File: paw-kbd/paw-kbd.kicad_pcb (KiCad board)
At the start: 2 copper layers, 30 parts, among them J1 OLED, J2 MJ-4PP-9, SW10 SW_PUSH, SW11 SW_PUSH, SW12 SW_PUSH, SW13 SW_PUSH, SW14 SW_PUSH, SW15 SW_PUSH, SW16 SW_PUSH, SW17 SW_PUSH, SW18 SW_PUSH, SW22 SW_PUSH, SW4 SW_PUSH, SW5 SW_PUSH, SW6 SW_PUSH, SW7 SW_PUSH, SW8 SW_PUSH, SW9 SW_PUSH, U1 ProMicro

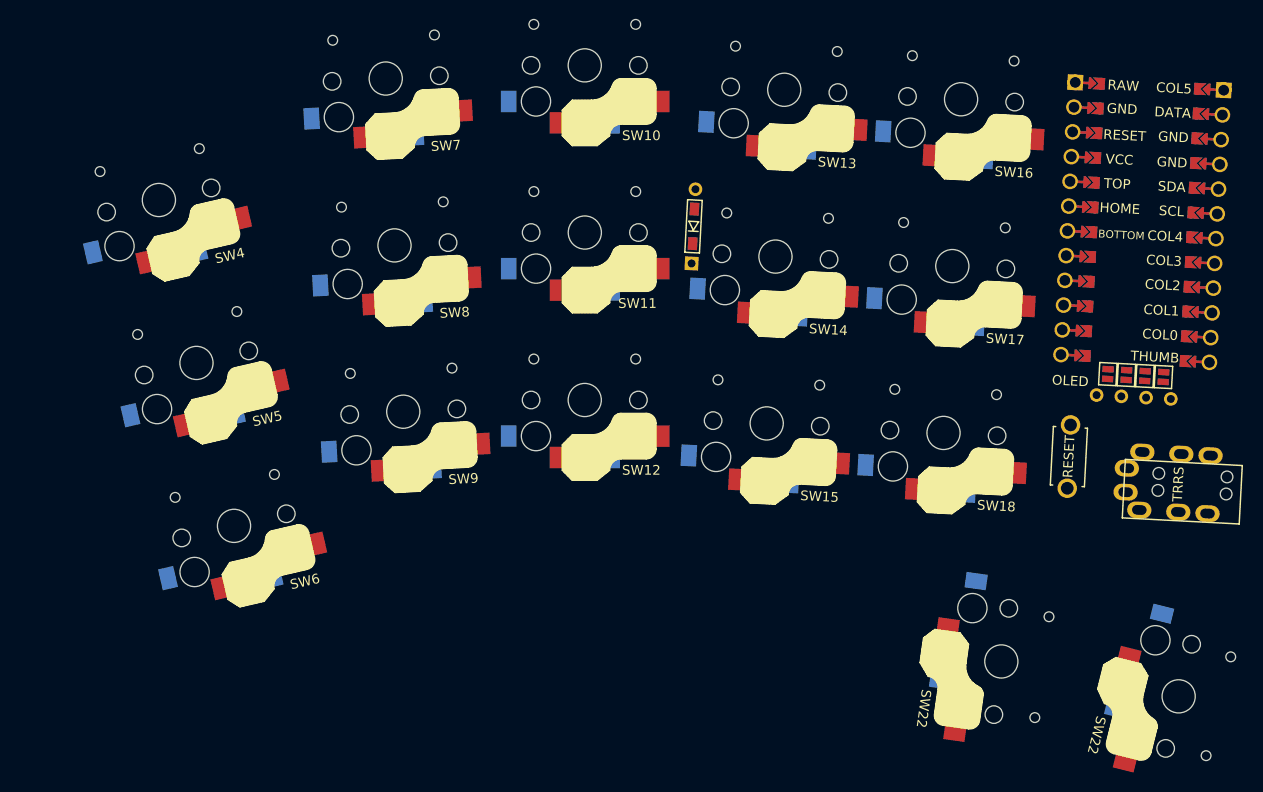
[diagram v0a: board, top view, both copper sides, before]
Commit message: schematic
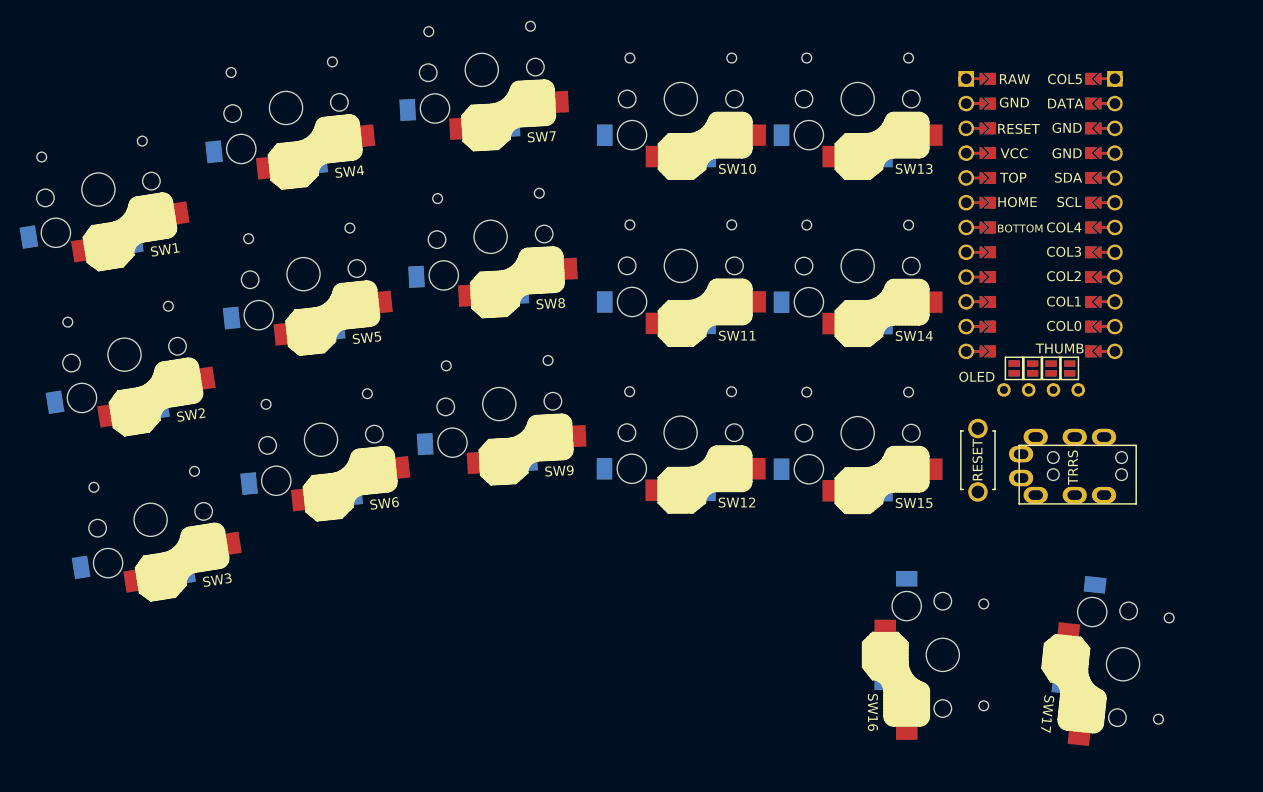
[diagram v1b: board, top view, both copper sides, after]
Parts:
- removed D14: DIODE, kbd:D3_TH_SMD
- SW1: renamed from SW4; footprint fp:ChocV1_V2_Hotswap_reversed_choc_spacing -> keeb-footprints:ChocV1_V2_Hotswap_reversed_choc_spacing
- SW10: renamed from SW13; footprint fp:ChocV1_V2_Hotswap_reversed_choc_spacing -> keeb-footprints:ChocV1_V2_Hotswap_reversed_choc_spacing
- SW11: renamed from SW14; footprint fp:ChocV1_V2_Hotswap_reversed_choc_spacing -> keeb-footprints:ChocV1_V2_Hotswap_reversed_choc_spacing
- SW12: renamed from SW15; footprint fp:ChocV1_V2_Hotswap_reversed_choc_spacing -> keeb-footprints:ChocV1_V2_Hotswap_reversed_choc_spacing
- SW13: renamed from SW16; footprint fp:ChocV1_V2_Hotswap_reversed_choc_spacing -> keeb-footprints:ChocV1_V2_Hotswap_reversed_choc_spacing
- SW14: renamed from SW17; footprint fp:ChocV1_V2_Hotswap_reversed_choc_spacing -> keeb-footprints:ChocV1_V2_Hotswap_reversed_choc_spacing
- SW15: renamed from SW18; footprint fp:ChocV1_V2_Hotswap_reversed_choc_spacing -> keeb-footprints:ChocV1_V2_Hotswap_reversed_choc_spacing
- SW2: renamed from SW5; footprint fp:ChocV1_V2_Hotswap_reversed_choc_spacing -> keeb-footprints:ChocV1_V2_Hotswap_reversed_choc_spacing
- SW3: renamed from SW6; footprint fp:ChocV1_V2_Hotswap_reversed_choc_spacing -> keeb-footprints:ChocV1_V2_Hotswap_reversed_choc_spacing
- SW4: renamed from SW7; footprint fp:ChocV1_V2_Hotswap_reversed_choc_spacing -> keeb-footprints:ChocV1_V2_Hotswap_reversed_choc_spacing
- SW5: renamed from SW8; footprint fp:ChocV1_V2_Hotswap_reversed_choc_spacing -> keeb-footprints:ChocV1_V2_Hotswap_reversed_choc_spacing
- SW6: renamed from SW9; footprint fp:ChocV1_V2_Hotswap_reversed_choc_spacing -> keeb-footprints:ChocV1_V2_Hotswap_reversed_choc_spacing
- SW7: renamed from SW10; footprint fp:ChocV1_V2_Hotswap_reversed_choc_spacing -> keeb-footprints:ChocV1_V2_Hotswap_reversed_choc_spacing
- SW8: renamed from SW11; footprint fp:ChocV1_V2_Hotswap_reversed_choc_spacing -> keeb-footprints:ChocV1_V2_Hotswap_reversed_choc_spacing
- SW9: renamed from SW12; footprint fp:ChocV1_V2_Hotswap_reversed_choc_spacing -> keeb-footprints:ChocV1_V2_Hotswap_reversed_choc_spacing
- moved J2 10.9 mm to (203.8, 102.5), turned to -90 degrees
- moved SW4 10.7 mm to (116.7, 64.9), turned to 6 degrees
- moved SW10 10.6 mm to (157.2, 64.0), turned to 0 degrees
- moved SW13 10.6 mm to (175.3, 64.0), turned to 0 degrees
- moved SW7 10.6 mm to (136.8, 61.0), turned to 3 degrees
- moved U1 10.5 mm to (194.1, 75.9), turned to 0 degrees
- moved SW5 9.78 mm to (118.5, 82.0), turned to 6 degrees
- moved SW11 9.75 mm to (157.2, 81.1), turned to 0 degrees
- moved SW14 9.70 mm to (175.3, 81.1), turned to 0 degrees
- moved SW8 9.67 mm to (137.7, 78.2), turned to 3 degrees
- moved JP4 9.65 mm to (197.0, 91.6), turned to -90 degrees
- moved JP5 9.65 mm to (197.0, 91.6), turned to -90 degrees
- moved JP3 9.64 mm to (195.1, 91.6), turned to -90 degrees
- moved JP6 9.64 mm to (195.1, 91.6), turned to -90 degrees
- moved JP2 9.63 mm to (193.2, 91.6), turned to -90 degrees
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- renumbered JP4 to JP1, JP3 to JP2, JP2 to JP3, JP1 to JP4, SW22 to SW16, SW22 to SW17
